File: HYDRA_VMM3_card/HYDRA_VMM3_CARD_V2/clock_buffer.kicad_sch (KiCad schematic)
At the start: 13 parts, among them U2 5PB1214CMGK8

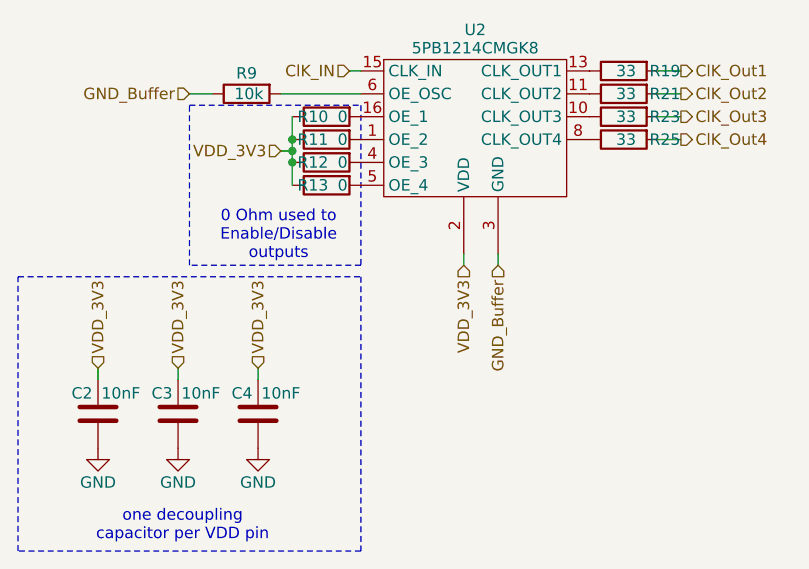
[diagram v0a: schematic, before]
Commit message: .
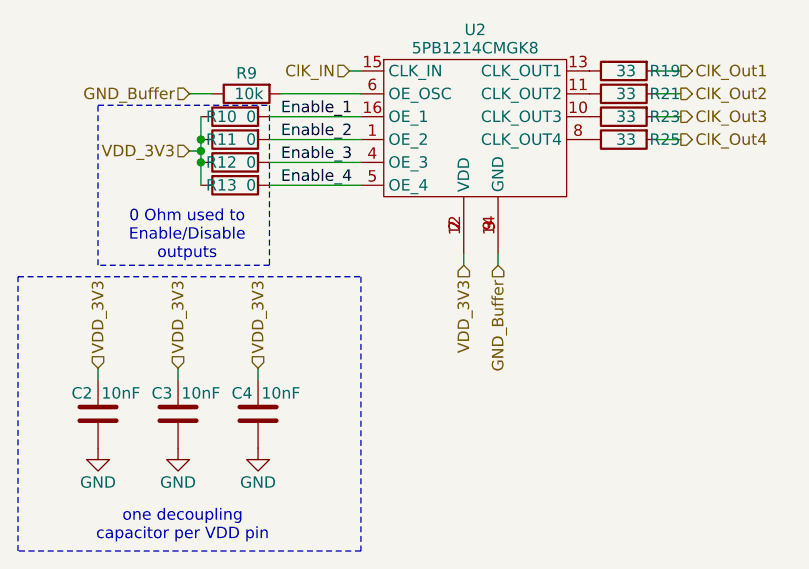
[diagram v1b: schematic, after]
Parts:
- C2, C3, C4: footprint Capacitor_SMD:C_0402_1005Metric -> Capacitor_SMD:C_0201_0603Metric
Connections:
- net GND_Buffer: now also U2.14 (GND), U2.9 (GND)
- net VDD_3V3: now also U2.12 (VDD), U2.7 (VDD)
- net Enable_3: now reaches R12.2, U2.4 (OE_3)
- net Enable_2: now reaches R11.2, U2.1 (OE_2)
- net Enable_1: now reaches R10.2, U2.16 (OE_1)
- net Enable_4: now reaches R13.2, U2.5 (OE_4)
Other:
- moved on the sheet: R10, R11, R12, R13
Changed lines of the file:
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@@
 	(paper "A4")
 	(junction
-		(at 121.92 95.25)
+		(at 111.76 95.25)
 		(diameter 0)
 		(color 0 0 0 0)
 	)
 	(junction
-		(at 121.92 92.71)
+		(at 111.76 92.71)
 		(diameter 0)
 		(color 0 0 0 0)
 	)
 	(junction
-		(at 121.92 93.98)
+		(at 111.76 93.98)
 		(diameter 0)
 		(color 0 0 0 0)
@@
 	(wire
 		(pts
-			(xy 121.92 90.17) (xy 121.92 92.71)
-		)
-		(stroke
-			(width 0)
-			(type default)
-		)
-	)
-	(wire
-		(pts
-			(xy 120.65 93.98) (xy 121.92 93.98)
+			(xy 111.76 90.17) (xy 111.76 92.71)
+		)
+		(stroke
+			(width 0)
+			(type default)
+		)
+	)
+	(wire
+		(pts
+			(xy 110.49 93.98) (xy 111.76 93.98)
 		)
 		(stroke
@@
 	(wire
 		(pts
+			(xy 119.38 90.17) (xy 129.54 90.17)
+		)
+		(stroke
+			(width 0)
+			(type default)
+		)
+	)
+	(wire
+		(pts
 			(xy 162.56 90.17) (xy 165.1 90.17)
 		)
@@
 	(wire
 		(pts
+			(xy 119.38 92.71) (xy 129.54 92.71)
+		)
+		(stroke
+			(width 0)
+			(type default)
+		)
+	)
+	(wire
+		(pts
 			(xy 162.56 87.63) (xy 165.1 87.63)
 		)
@@
 	(wire
 		(pts
-			(xy 121.92 93.98) (xy 121.92 95.25)
+			(xy 119.38 97.79) (xy 129.54 97.79)
+		)
+		(stroke
+			(width 0)
+			(type default)
+		)
+	)
+	(wire
+		(pts
+			(xy 111.76 93.98) (xy 111.76 95.25)
+		)
+		(stroke
+			(width 0)
+			(type default)
+		)
+	)
+	(wire
+		(pts
+			(xy 119.38 95.25) (xy 129.54 95.25)
 		)
 		(stroke
@@
 	(wire
 		(pts
-			(xy 121.92 95.25) (xy 121.92 97.79)
+			(xy 111.76 95.25) (xy 111.76 97.79)
 		)
 		(stroke
@@
 	(wire
 		(pts
-			(xy 121.92 92.71) (xy 121.92 93.98)
+			(xy 111.76 92.71) (xy 111.76 93.98)
 		)
 		(stroke
@@
 	)
 	(rectangle
-		(start 110.49 88.9)
-		(end 129.54 106.68)
+		(start 100.33 88.9)
+		(end 119.38 106.68)
 		(stroke
 			(width 0)
@@
 	(text "0 Ohm used to \nEnable/Disable\noutputs"
 		(exclude_from_sim no)
-		(at 120.396 103.378 0)
-		(effects
-			(font
-				(size 1.27 1.27)
-			)
+		(at 110.236 103.378 0)
+		(effects
+			(font
+				(size 1.27 1.27)
+			)
+		)
+	)
+	(label "Enable_4"
+		(at 120.65 97.79 0)
+		(fields_autoplaced yes)
+		(effects
+			(font
+				(size 1.27 1.27)
+			)
+			(justify left bottom)
+		)
+	)
+	(label "Enable_1"
+		(at 120.65 90.17 0)
+		(fields_autoplaced yes)
+		(effects
+			(font
+				(size 1.27 1.27)
+			)
+			(justify left bottom)
+		)
+	)
+	(label "Enable_3"
+		(at 120.65 95.25 0)
+		(fields_autoplaced yes)
+		(effects
+			(font
+				(size 1.27 1.27)
+			)
+			(justify left bottom)
+		)
+	)
+	(label "Enable_2"
+		(at 120.65 92.71 0)
+		(fields_autoplaced yes)
+		(effects
+			(font
+				(size 1.27 1.27)
+			)
+			(justify left bottom)
 		)
 	)
@@
 	(hierarchical_label "VDD_3V3"
 		(shape input)
-		(at 120.65 93.98 180)
+		(at 110.49 93.98 180)
 		(fields_autoplaced yes)
 		(effects
@@
 	(symbol
 		(lib_id "Device:R")
-		(at 125.73 95.25 90)
+		(at 115.57 95.25 90)
 		(mirror x)
 		(unit 1)
@@
 		(dnp no)
 		(property "Reference" "R12"
-			(at 124.206 95.25 90)
+			(at 114.046 95.25 90)
 			(effects
 				(font
@@
 		)
 		(property "Value" "0"
-			(at 127.508 95.25 90)
+			(at 117.348 95.25 90)
 			(effects
 				(font
@@
 		)
 		(property "Footprint" "Resistor_SMD:R_0201_0603Metric"
-			(at 125.73 93.472 90)
+			(at 115.57 93.472 90)
 			(effects
 				(font
@@
 		)
 		(property "Datasheet" "~"
-			(at 125.73 95.25 0)
+			(at 115.57 95.25 0)
 			(effects
 				(font
@@
 		)
 		(property "Description" "Resistor"
-			(at 125.73 95.25 0)
+			(at 115.57 95.25 0)
 			(effects
 				(font
@@
 	(symbol
 		(lib_id "Device:R")
-		(at 125.73 92.71 90)
+		(at 115.57 92.71 90)
 		(mirror x)
 		(unit 1)
@@
 		(dnp no)
 		(property "Reference" "R11"
-			(at 124.206 92.71 90)
+			(at 114.046 92.71 90)
 			(effects
 				(font
@@
 		)
 		(property "Value" "0"
-			(at 127.508 92.71 90)
+			(at 117.348 92.71 90)
 			(effects
 				(font
@@
 		)
 		(property "Footprint" "Resistor_SMD:R_0201_0603Metric"
-			(at 125.73 90.932 90)
+			(at 115.57 90.932 90)
 			(effects
 				(font
@@
 		)
 		(property "Datasheet" "~"
-			(at 125.73 92.71 0)
+			(at 115.57 92.71 0)
 			(effects
 				(font
@@
 		)
 		(property "Description" "Resistor"
-			(at 125.73 92.71 0)
+			(at 115.57 92.71 0)
 			(effects
 				(font
@@
 			)
 		)
-		(property "Footprint" "Capacitor_SMD:C_0402_1005Metric"
+		(property "Footprint" "Capacitor_SMD:C_0201_0603Metric"
 			(at 99.3648 119.38 0)
 			(effects
@@
 	(symbol
 		(lib_id "Device:R")
-		(at 125.73 90.17 90)
+		(at 115.57 90.17 90)
 		(mirror x)
 		(unit 1)
@@
 		(dnp no)
 		(property "Reference" "R10"
-			(at 124.206 90.17 90)
+			(at 114.046 90.17 90)
 			(effects
 				(font
@@
 		)
 		(property "Value" "0"
-			(at 127.508 90.17 90)
+			(at 117.348 90.17 90)
 			(effects
 				(font
@@
 		)
 		(property "Footprint" "Resistor_SMD:R_0201_0603Metric"
-			(at 125.73 88.392 90)
+			(at 115.57 88.392 90)
 			(effects
 				(font
@@
 		)
 		(property "Datasheet" "~"
-			(at 125.73 90.17 0)
+			(at 115.57 90.17 0)
 			(effects
 				(font
@@
 		)
 		(property "Description" "Resistor"
-			(at 125.73 90.17 0)
+			(at 115.57 90.17 0)
 			(effects
 				(font
@@
 	(symbol
 		(lib_id "Device:R")
-		(at 125.73 97.79 90)
+		(at 115.57 97.79 90)
 		(mirror x)
 		(unit 1)
@@
 		(dnp no)
 		(property "Reference" "R13"
-			(at 124.206 97.79 90)
+			(at 114.046 97.79 90)
 			(effects
 				(font
@@
 		)
 		(property "Value" "0"
-			(at 127.508 97.79 90)
+			(at 117.348 97.79 90)
 			(effects
 				(font
@@
 		)
 		(property "Footprint" "Resistor_SMD:R_0201_0603Metric"
-			(at 125.73 96.012 90)
+			(at 115.57 96.012 90)
 			(effects
 				(font
@@
 		)
 		(property "Datasheet" "~"
-			(at 125.73 97.79 0)
+			(at 115.57 97.79 0)
 			(effects
 				(font
@@
 		)
 		(property "Description" "Resistor"
-			(at 125.73 97.79 0)
+			(at 115.57 97.79 0)
 			(effects
 				(font
@@
 		(pin "10"
 		)
+		(pin "7"
+		)
+		(pin "12"
+		)
+		(pin "14"
+		)
+		(pin "9"
+		)
 		(instances
 			(project ""
@@
 			)
 		)
-		(property "Footprint" "Capacitor_SMD:C_0402_1005Metric"
+		(property "Footprint" "Capacitor_SMD:C_0201_0603Metric"
 			(at 117.1448 119.38 0)
 			(effects
@@
 			)
 		)
-		(property "Footprint" "Capacitor_SMD:C_0402_1005Metric"
+		(property "Footprint" "Capacitor_SMD:C_0201_0603Metric"
 			(at 108.2548 119.38 0)
 			(effects
